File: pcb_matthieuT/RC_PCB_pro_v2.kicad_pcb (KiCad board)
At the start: 2 copper layers, 100 x 70 mm, 14 parts

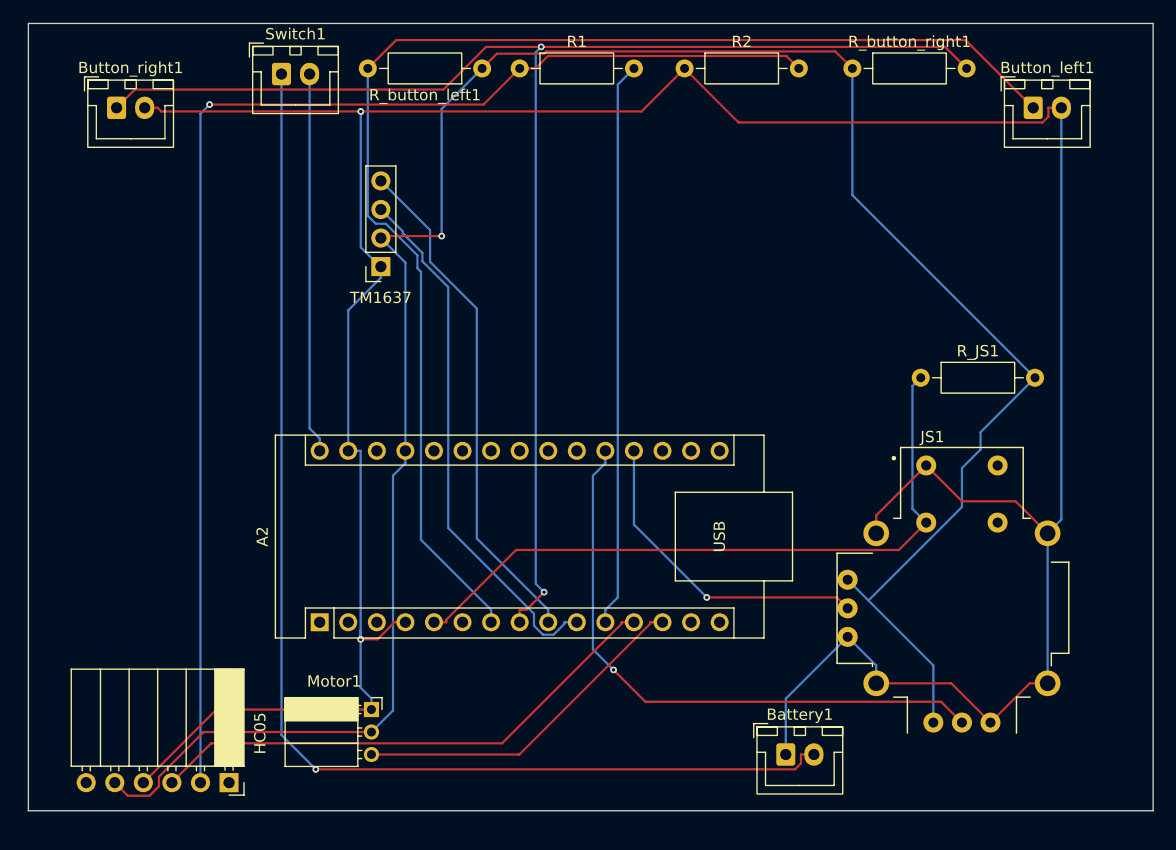
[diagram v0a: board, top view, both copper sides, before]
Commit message: Remote PCB V2
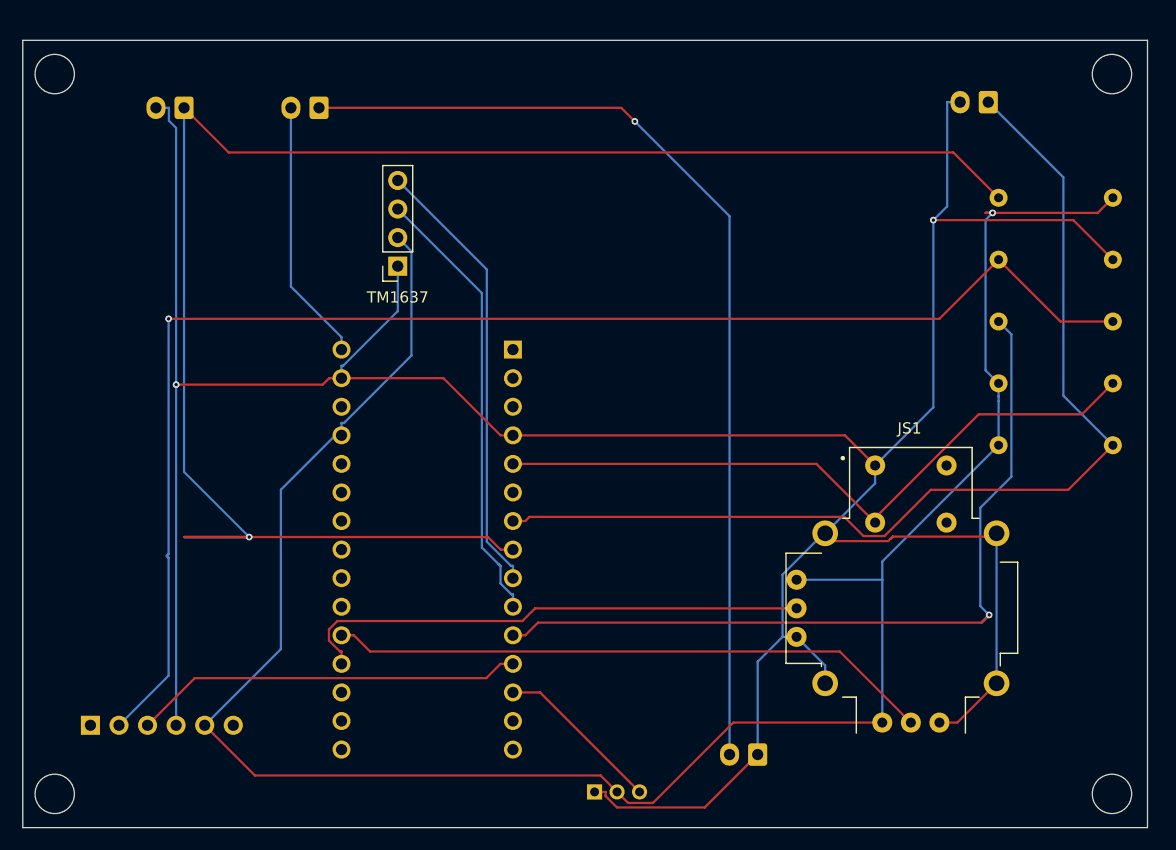
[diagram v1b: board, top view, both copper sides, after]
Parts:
- A2, Battery1, Button_left1, Button_right1, HC05, Motor1, R1, R2, R_JS1, R_button_left1, R_button_right1, Switch1: moved to B.Cu
- moved R1 57.3 mm to (196.6, 77.0), turned to 180 degrees
- moved R_button_left1 56.8 mm to (186.4, 88.0), turned to 0 degrees
- moved R2 41.7 mm to (196.6, 71.5), turned to 180 degrees
- moved A2 29.7 mm to (143.2, 79.5), turned to 180 degrees
- moved R_button_right1 25.9 mm to (196.6, 66.0), turned to 180 degrees
- moved Motor1 21.1 mm to (150.5, 118.8), turned to -90 degrees
- moved R_JS1 17.1 mm to (196.6, 82.5), turned to 180 degrees
- moved HC05 13.3 mm to (105.7, 112.9)
- moved Button_right1 6.00 mm to (114.0, 58.0), turned to 180 degrees
- moved JS1 4.54 mm to (178.6, 102.5)
- moved Switch1 4.49 mm to (126.0, 58.0), turned to 180 degrees
- moved Button_left1 4.03 mm to (185.5, 57.5), turned to 180 degrees
- moved Battery1 2.50 mm to (165.0, 115.5), turned to 180 degrees
- moved TM1637 1.50 mm to (133.0, 72.1)
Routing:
- net /Button2: track 131.5 -> 163.4 mm, vias 2 -> 1
- net /Button1: track 117.0 -> 92.6 mm
- net /RX: track 50.3 -> 73.1 mm, vias 0 -> 1
- net Net-(Battery1-Pin_2): track 108.4 -> 88.4 mm
- net /JS_V: track 28.6 -> 46.0 mm, vias 1 -> 0
- net /Haptic: track 30.8 -> 14.9 mm
- net +5V: track 204.3 -> 189.9 mm
- net /TX: track 47.1 -> 34.7 mm
- net Net-(HC05-Pin_2): track 115.3 -> 126.7 mm
- net /Power: track 33.9 -> 23.4 mm
- net /DIO: track 47.6 -> 39.9 mm
- net /Clock: track 45.4 -> 39.7 mm
- net GND: track 279.9 -> 277.2 mm
- net /Button_JS: track 61.3 -> 60.8 mm
- net /JS_H: track 53.6 -> 53.8 mm, vias 1 -> 0
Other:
- outline, holes or cut-outs redrawn
- board text added: "+"
- board text added: "-"
- board text added: "1 kΩ"
- board text added: "47 kΩ"
- board text added: "470 kΩ"
